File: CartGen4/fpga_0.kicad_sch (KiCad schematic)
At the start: 12 parts, among them U9 LFXP2-8E-5MN132C

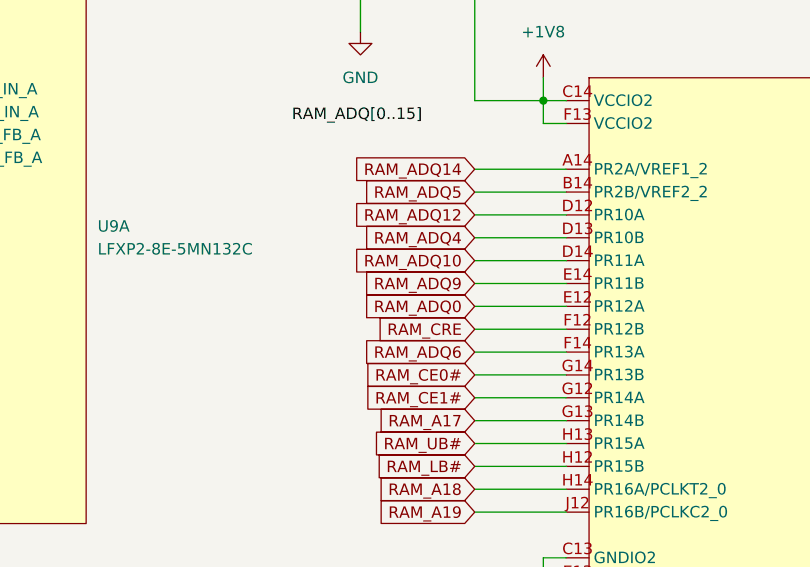
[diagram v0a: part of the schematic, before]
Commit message: Started routing more ram, but I'd better sleep...
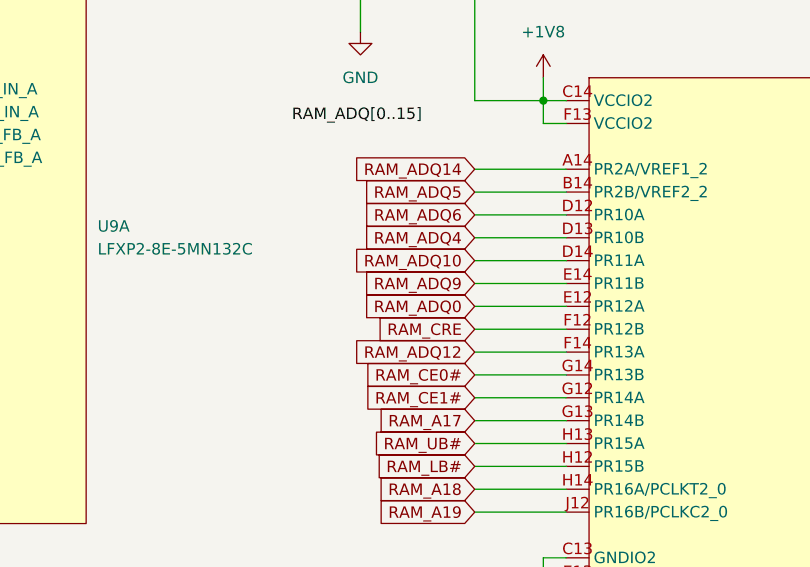
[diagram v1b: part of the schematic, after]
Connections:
- net RAM_ADQ12: now also U9.F14 (PR13A); no longer U9.D12 (PR10A)
- net RAM_ADQ6: now also U9.D12 (PR10A); no longer U9.F14 (PR13A)
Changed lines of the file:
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@@
-    )
-  )
-  (global_label "RAM_ADQ12" (shape input) (at 217.1625 57.15 180) (fields_autoplaced)
-    (effects (font (size 1.27 1.27)) (justify right))
-    (property "Intersheet References" "${INTERSHEET_REFS}" (id 0) (at 203.8637 57.0706 0)
-      (effects (font (size 1.27 1.27)) (justify right) hide)
     )
   )
@@
     )
   )
+  (global_label "RAM_ADQ6" (shape input) (at 217.17 57.15 180) (fields_autoplaced)
+    (effects (font (size 1.27 1.27)) (justify right))
+    (property "Intersheet References" "${INTERSHEET_REFS}" (id 0) (at 205.0807 57.0706 0)
+      (effects (font (size 1.27 1.27)) (justify right) hide)
+    )
+  )
   (global_label "PS_PGOOD" (shape input) (at 53.34 87.63 180) (fields_autoplaced)
     (effects (font (size 1.27 1.27)) (justify right))
@@
     (effects (font (size 1.27 1.27)) (justify right))
     (property "Intersheet References" "${INTERSHEET_REFS}" (id 0) (at 205.0732 59.6106 0)
+      (effects (font (size 1.27 1.27)) (justify right) hide)
+    )
+  )
+  (global_label "RAM_ADQ12" (shape input) (at 217.1625 72.39 180) (fields_autoplaced)
+    (effects (font (size 1.27 1.27)) (justify right))
+    (property "Intersheet References" "${INTERSHEET_REFS}" (id 0) (at 203.8637 72.3106 0)
       (effects (font (size 1.27 1.27)) (justify right) hide)
     )
@@
       (effects (font (size 1.27 1.27)) (justify right) hide)
     )
-  )
-  (global_label "RAM_ADQ6" (shape input) (at 217.1625 72.39 180) (fields_autoplaced)
-    (effects (font (size 1.27 1.27)) (justify right))
-    (property "Intersheet References" "${INTERSHEET_REFS}" (id 0) (at 205.0732 72.3106 0)
-      (effects (font (size 1.27 1.27)) (justify right) hide)
-    )

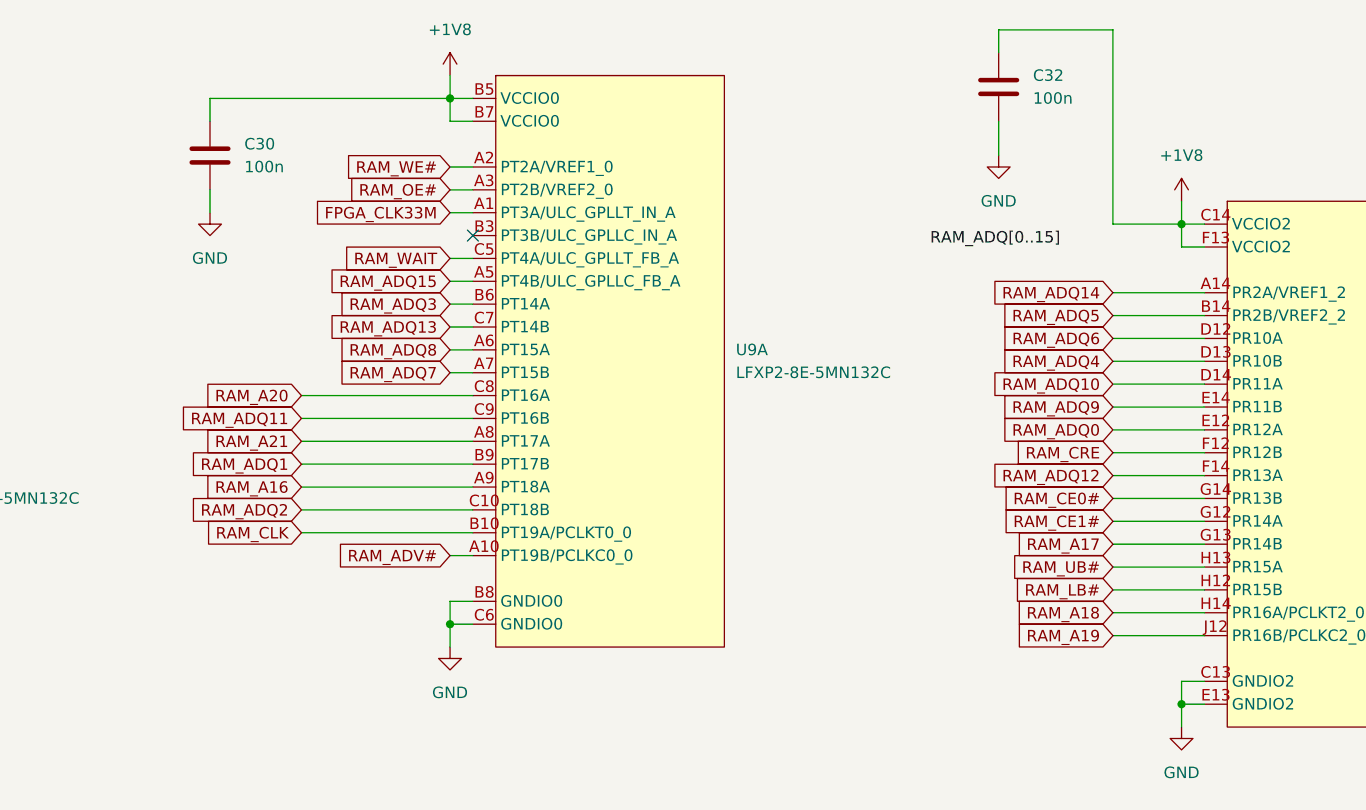
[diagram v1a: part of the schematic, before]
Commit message: More RAM wire changes (i wanna cry)
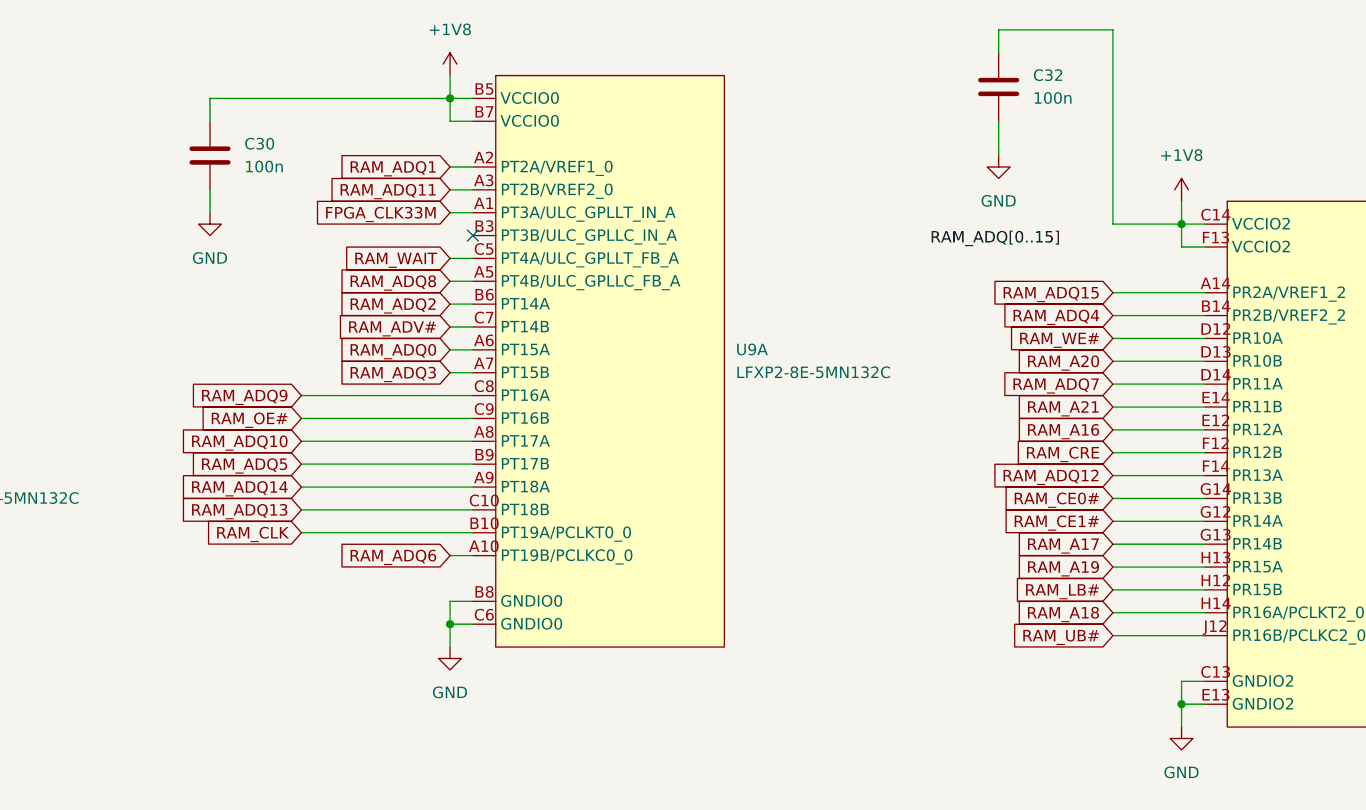
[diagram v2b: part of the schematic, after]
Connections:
- net RAM_A16: now also U9.E12 (PR12A); no longer U9.A9 (PT18A)
- net RAM_A19: now also U9.H13 (PR15A); no longer U9.J12 (PR16B/PCLKC2_0)
- net RAM_A20: now also U9.D13 (PR10B); no longer U9.C8 (PT16A)
- net RAM_A21: now also U9.E14 (PR11B); no longer U9.A8 (PT17A)
- net RAM_ADQ0: now also U9.A6 (PT15A); no longer U9.E12 (PR12A)
- net RAM_ADQ1: now also U9.A2 (PT2A/VREF1_0); no longer U9.B9 (PT17B)
- net RAM_ADQ10: now also U9.A8 (PT17A); no longer U9.D14 (PR11A)
- net RAM_ADQ11: now also U9.A3 (PT2B/VREF2_0); no longer U9.C9 (PT16B)
- net RAM_ADQ13: now also U9.C10 (PT18B); no longer U9.C7 (PT14B)
- net RAM_ADQ14: now also U9.A9 (PT18A); no longer U9.A14 (PR2A/VREF1_2)
- net RAM_ADQ15: now also U9.A14 (PR2A/VREF1_2); no longer U9.A5 (PT4B/ULC_GPLLC_FB_A)
- net RAM_ADQ2: now also U9.B6 (PT14A); no longer U9.C10 (PT18B)
- net RAM_ADQ3: now also U9.A7 (PT15B); no longer U9.B6 (PT14A)
- net RAM_ADQ4: now also U9.B14 (PR2B/VREF2_2); no longer U9.D13 (PR10B)
- net RAM_ADQ5: now also U9.B9 (PT17B); no longer U9.B14 (PR2B/VREF2_2)
- net RAM_ADQ6: now also U9.A10 (PT19B/PCLKC0_0); no longer U9.D12 (PR10A)
- net RAM_ADQ7: now also U9.D14 (PR11A); no longer U9.A7 (PT15B)
- net RAM_ADQ8: now also U9.A5 (PT4B/ULC_GPLLC_FB_A); no longer U9.A6 (PT15A)
- net RAM_ADQ9: now also U9.C8 (PT16A); no longer U9.E14 (PR11B)
- net RAM_ADV#: now also U9.C7 (PT14B); no longer U9.A10 (PT19B/PCLKC0_0)
- net RAM_OE#: now also U9.C9 (PT16B); no longer U9.A3 (PT2B/VREF2_0)
- net RAM_UB#: now also U9.J12 (PR16B/PCLKC2_0); no longer U9.H13 (PR15A)
- net RAM_WE#: now also U9.D12 (PR10A); no longer U9.A2 (PT2A/VREF1_0)
